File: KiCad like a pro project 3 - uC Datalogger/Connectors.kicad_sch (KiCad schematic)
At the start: 4 parts, among them J1 Conn_01x04_Male, J2 Conn_01x09_Male, J3 Conn_01x04_Male, J4 Conn_02x03_Odd_Even

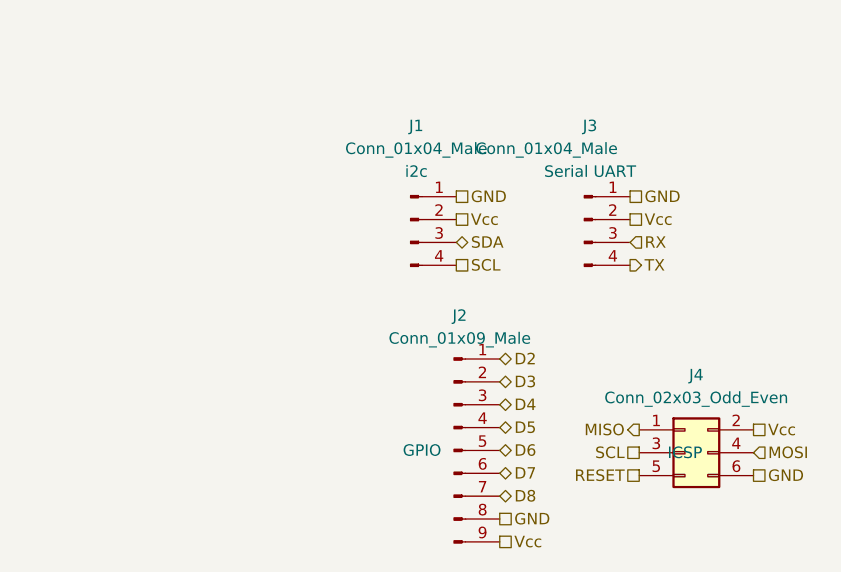
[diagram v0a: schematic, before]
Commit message: enh layout and text schematic
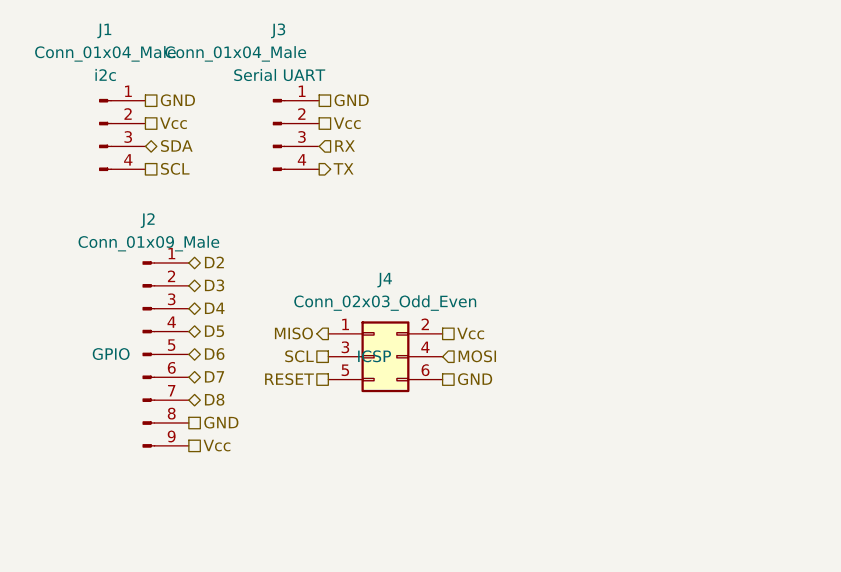
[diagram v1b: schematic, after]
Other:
- title: (none) -> Connectors
- moved on the sheet: J1, J2, J3, J4
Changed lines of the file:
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@@
 (kicad_sch (version 20211123) (generator eeschema)
   (paper "A4")
-  (hierarchical_label "D7" (shape bidirectional) (at 181.864 127.508 0)
+  (title_block
+    (title "Connectors")
+    (date "2022-07-31")
+    (rev "V1.0")
+    (comment 1 "Casper Tak")
+  )
+  (hierarchical_label "D7" (shape bidirectional) (at 147.32 116.84 0)
     (effects (font (size 1.27 1.27)) (justify left))
   )
-  (hierarchical_label "RESET" (shape passive) (at 197.358 127.762 180)
+  (hierarchical_label "RESET" (shape passive) (at 162.814 117.094 180)
     (effects (font (size 1.27 1.27)) (justify right))
   )
-  (hierarchical_label "RX" (shape input) (at 196.342 101.854 0)
+  (hierarchical_label "RX" (shape input) (at 161.798 91.186 0)
     (effects (font (size 1.27 1.27)) (justify left))
   )
-  (hierarchical_label "TX" (shape output) (at 196.342 104.394 0)
+  (hierarchical_label "TX" (shape output) (at 161.798 93.726 0)
     (effects (font (size 1.27 1.27)) (justify left))
   )
-  (hierarchical_label "SCL" (shape passive) (at 177.038 104.394 0)
+  (hierarchical_label "SCL" (shape passive) (at 142.494 93.726 0)
     (effects (font (size 1.27 1.27)) (justify left))
   )
-  (hierarchical_label "D5" (shape bidirectional) (at 181.864 122.428 0)
+  (hierarchical_label "D5" (shape bidirectional) (at 147.32 111.76 0)
     (effects (font (size 1.27 1.27)) (justify left))
   )
-  (hierarchical_label "D4" (shape bidirectional) (at 181.864 119.888 0)
+  (hierarchical_label "D4" (shape bidirectional) (at 147.32 109.22 0)
     (effects (font (size 1.27 1.27)) (justify left))
   )
-  (hierarchical_label "SDA" (shape bidirectional) (at 177.038 101.854 0)
+  (hierarchical_label "SDA" (shape bidirectional) (at 142.494 91.186 0)
     (effects (font (size 1.27 1.27)) (justify left))
   )
-  (hierarchical_label "GND" (shape passive) (at 196.342 96.774 0)
+  (hierarchical_label "GND" (shape passive) (at 161.798 86.106 0)
     (effects (font (size 1.27 1.27)) (justify left))
   )
-  (hierarchical_label "GND" (shape passive) (at 177.038 96.774 0)
+  (hierarchical_label "GND" (shape passive) (at 142.494 86.106 0)
     (effects (font (size 1.27 1.27)) (justify left))
   )
-  (hierarchical_label "D8" (shape bidirectional) (at 181.864 130.048 0)
+  (hierarchical_label "D8" (shape bidirectional) (at 147.32 119.38 0)
     (effects (font (size 1.27 1.27)) (justify left))
   )
-  (hierarchical_label "SCL" (shape passive) (at 197.358 125.222 180)
+  (hierarchical_label "SCL" (shape passive) (at 162.814 114.554 180)
     (effects (font (size 1.27 1.27)) (justify right))
   )
-  (hierarchical_label "GND" (shape passive) (at 181.864 132.588 0)
+  (hierarchical_label "GND" (shape passive) (at 147.32 121.92 0)
     (effects (font (size 1.27 1.27)) (justify left))
   )
-  (hierarchical_label "Vcc" (shape passive) (at 196.342 99.314 0)
+  (hierarchical_label "Vcc" (shape passive) (at 161.798 88.646 0)
     (effects (font (size 1.27 1.27)) (justify left))
   )
-  (hierarchical_label "Vcc" (shape passive) (at 210.058 122.682 0)
+  (hierarchical_label "Vcc" (shape passive) (at 175.514 112.014 0)
     (effects (font (size 1.27 1.27)) (justify left))
   )
-  (hierarchical_label "Vcc" (shape passive) (at 177.038 99.314 0)
+  (hierarchical_label "Vcc" (shape passive) (at 142.494 88.646 0)
     (effects (font (size 1.27 1.27)) (justify left))
   )
-  (hierarchical_label "GND" (shape passive) (at 210.058 127.762 0)
+  (hierarchical_label "GND" (shape passive) (at 175.514 117.094 0)
     (effects (font (size 1.27 1.27)) (justify left))
   )
-  (hierarchical_label "MISO" (shape output) (at 197.358 122.682 180)
+  (hierarchical_label "MISO" (shape output) (at 162.814 112.014 180)
     (effects (font (size 1.27 1.27)) (justify right))
   )
-  (hierarchical_label "D3" (shape bidirectional) (at 181.864 117.348 0)
+  (hierarchical_label "D3" (shape bidirectional) (at 147.32 106.68 0)
     (effects (font (size 1.27 1.27)) (justify left))
   )
-  (hierarchical_label "Vcc" (shape passive) (at 181.864 135.128 0)
+  (hierarchical_label "Vcc" (shape passive) (at 147.32 124.46 0)
     (effects (font (size 1.27 1.27)) (justify left))
   )
-  (hierarchical_label "D2" (shape bidirectional) (at 181.864 114.808 0)
+  (hierarchical_label "D2" (shape bidirectional) (at 147.32 104.14 0)
     (effects (font (size 1.27 1.27)) (justify left))
   )
-  (hierarchical_label "D6" (shape bidirectional) (at 181.864 124.968 0)
+  (hierarchical_label "D6" (shape bidirectional) (at 147.32 114.3 0)
     (effects (font (size 1.27 1.27)) (justify left))
   )
-  (hierarchical_label "MOSI" (shape input) (at 210.058 125.222 0)
+  (hierarchical_label "MOSI" (shape input) (at 175.514 114.554 0)
     (effects (font (size 1.27 1.27)) (justify left))
   )
-  (symbol (lib_id "Connector_Generic:Conn_02x03_Odd_Even") (at 202.438 125.222 0) (unit 1)
+  (symbol (lib_id "Connector_Generic:Conn_02x03_Odd_Even") (at 167.894 114.554 0) (unit 1)
     (in_bom yes) (on_board yes)
-    (property "Reference" "J4" (id 0) (at 203.708 116.586 0))
-    (property "Value" "Conn_02x03_Odd_Even" (id 1) (at 203.708 119.126 0))
-    (property "Footprint" "Connector_PinHeader_2.54mm:PinHeader_2x03_P2.54mm_Vertical" (id 2) (at 202.438 125.222 0)
+    (property "Reference" "J4" (id 0) (at 169.164 105.918 0))
+    (property "Value" "Conn_02x03_Odd_Even" (id 1) (at 169.164 108.458 0))
+    (property "Footprint" "Connector_PinHeader_2.54mm:PinHeader_2x03_P2.54mm_Vertical" (id 2) (at 167.894 114.554 0)
       (effects (font (size 1.27 1.27)) hide)
     )
-    (property "Datasheet" "~" (id 3) (at 202.438 125.222 0)
+    (property "Datasheet" "~" (id 3) (at 167.894 114.554 0)
       (effects (font (size 1.27 1.27)) hide)
     )
-    (property "Purpose" "ICSP" (id 4) (at 202.438 125.222 0))
+    (property "Purpose" "ICSP" (id 4) (at 167.894 114.554 0))
     (pin "1")
     (pin "2")
@@
     (pin "6")
   )
-  (symbol (lib_id "Connector:Conn_01x09_Male") (at 176.784 124.968 0) (unit 1)
+  (symbol (lib_id "Connector:Conn_01x09_Male") (at 142.24 114.3 0) (unit 1)
     (in_bom yes) (on_board yes)
-    (property "Reference" "J2" (id 0) (at 177.419 109.982 0))
-    (property "Value" "Conn_01x09_Male" (id 1) (at 177.419 112.522 0))
-    (property "Footprint" "Connector_PinHeader_2.54mm:PinHeader_1x09_P2.54mm_Vertical" (id 2) (at 176.784 124.968 0)
+    (property "Reference" "J2" (id 0) (at 142.875 99.314 0))
+    (property "Value" "Conn_01x09_Male" (id 1) (at 142.875 101.854 0))
+    (property "Footprint" "Connector_PinHeader_2.54mm:PinHeader_1x09_P2.54mm_Vertical" (id 2) (at 142.24 114.3 0)
       (effects (font (size 1.27 1.27)) hide)
     )
-    (property "Datasheet" "~" (id 3) (at 176.784 124.968 0)
+    (property "Datasheet" "~" (id 3) (at 142.24 114.3 0)
       (effects (font (size 1.27 1.27)) hide)
     )
-    (property "Purpose" "GPIO" (id 4) (at 173.228 124.968 0))
+    (property "Purpose" "GPIO" (id 4) (at 138.684 114.3 0))
     (pin "1")
     (pin "2")
@@
     (pin "9")
   )
-  (symbol (lib_id "Connector:Conn_01x04_Male") (at 191.262 99.314 0) (unit 1)
+  (symbol (lib_id "Connector:Conn_01x04_Male") (at 156.718 88.646 0) (unit 1)
     (in_bom yes) (on_board yes)
-    (property "Reference" "J3" (id 0) (at 191.897 88.9 0))
-    (property "Value" "Conn_01x04_Male" (id 1) (at 187.071 91.44 0))
-    (property "Footprint" "Connector_PinHeader_2.54mm:PinHeader_1x04_P2.54mm_Vertical" (id 2) (at 191.262 99.314 0)
+    (property "Reference" "J3" (id 0) (at 157.353 78.232 0))
+    (property "Value" "Conn_01x04_Male" (id 1) (at 152.527 80.772 0))
+    (property "Footprint" "Connector_PinHeader_2.54mm:PinHeader_1x04_P2.54mm_Vertical" (id 2) (at 156.718 88.646 0)
       (effects (font (size 1.27 1.27)) hide)
     )
-    (property "Datasheet" "~" (id 3) (at 191.262 99.314 0)
+    (property "Datasheet" "~" (id 3) (at 156.718 88.646 0)
       (effects (font (size 1.27 1.27)) hide)
     )
-    (property "Purpose" "Serial UART" (id 4) (at 191.897 93.98 0))
+    (property "Purpose" "Serial UART" (id 4) (at 157.353 83.312 0))
     (pin "1")
     (pin "2")
@@
     (pin "4")
   )
-  (symbol (lib_id "Connector:Conn_01x04_Male") (at 171.958 99.314 0) (unit 1)
+  (symbol (lib_id "Connector:Conn_01x04_Male") (at 137.414 88.646 0) (unit 1)
     (in_bom yes) (on_board yes) (fields_autoplaced)
-    (property "Reference" "J1" (id 0) (at 172.593 88.9 0))
-    (property "Value" "Conn_01x04_Male" (id 1) (at 172.593 91.44 0))
-    (property "Footprint" "Connector_PinHeader_2.54mm:PinHeader_1x04_P2.54mm_Vertical" (id 2) (at 171.958 99.314 0)
+    (property "Reference" "J1" (id 0) (at 138.049 78.232 0))
+    (property "Value" "Conn_01x04_Male" (id 1) (at 138.049 80.772 0))
+    (property "Footprint" "Connector_PinHeader_2.54mm:PinHeader_1x04_P2.54mm_Vertical" (id 2) (at 137.414 88.646 0)
       (effects (font (size 1.27 1.27)) hide)
     )
-    (property "Datasheet" "~" (id 3) (at 171.958 99.314 0)
+    (property "Datasheet" "~" (id 3) (at 137.414 88.646 0)
       (effects (font (size 1.27 1.27)) hide)
     )
-    (property "Purpose" "i2c" (id 4) (at 172.593 93.98 0))
+    (property "Purpose" "i2c" (id 4) (at 138.049 83.312 0))
     (pin "1")
     (pin "2")
